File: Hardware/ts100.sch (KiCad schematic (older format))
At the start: 46 parts, among them J1 Jack-DC, J2 Iron+, J3 Iron-, J4 GND, J5 SWD, Q1 2SC3356, Q2 IRF4905STRLPBF, SW1 SW_Push, SW2 SW_Push, U1 AD823, U2 EUP3476, U3 1N4728A, U4 128x32 OLED, U5 STM32F103C8T6, Y1 8M

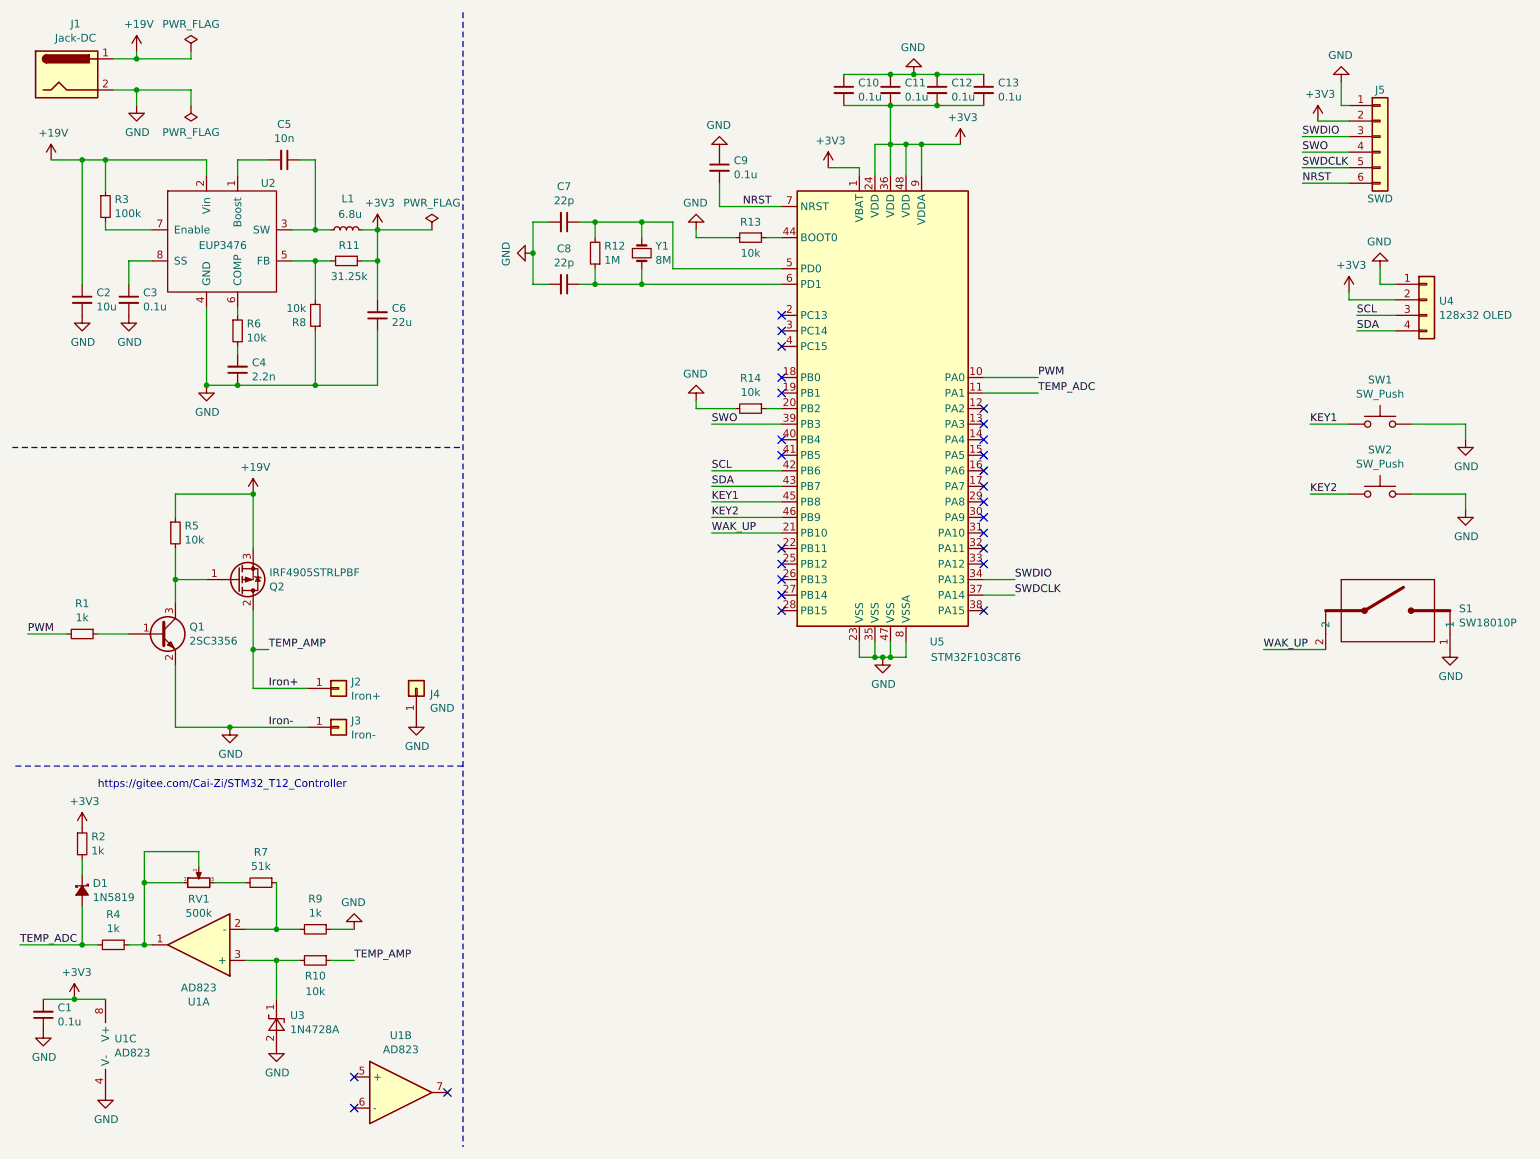
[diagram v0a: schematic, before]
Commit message: 修改原理图
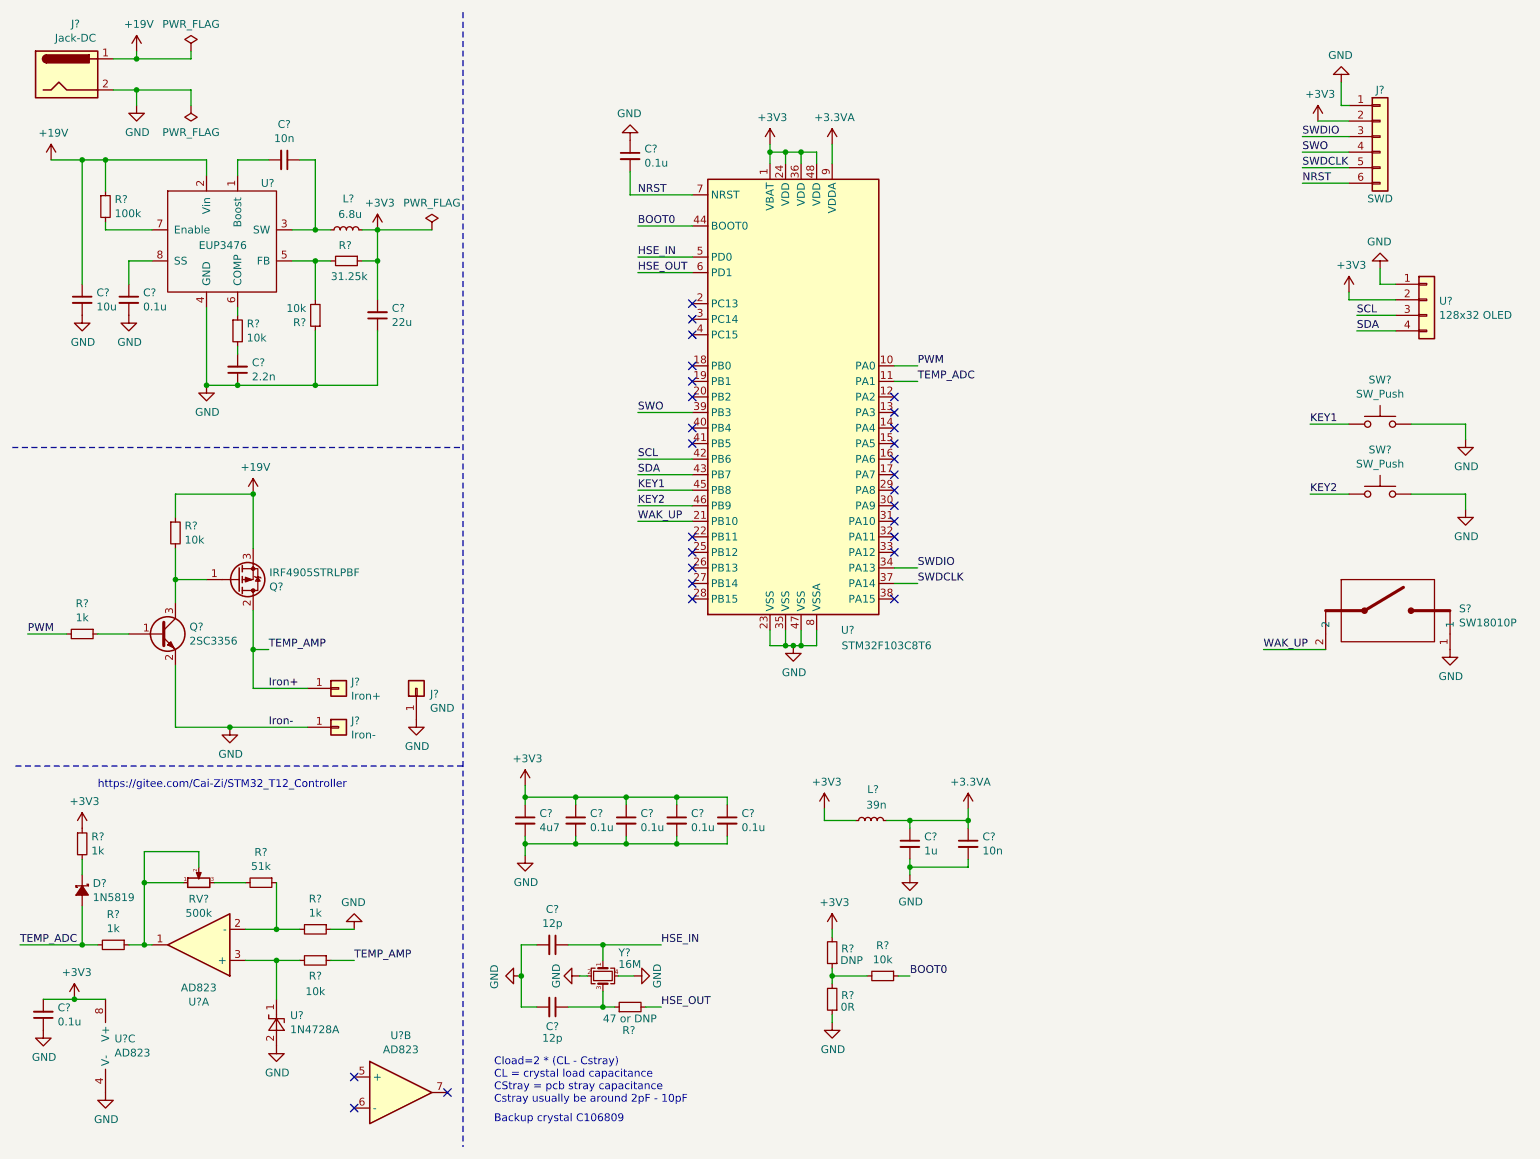
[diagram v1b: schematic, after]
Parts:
- removed R13: 10k, Resistor_SMD:R_0603_1608Metric, symbol Device:R_Small
- removed Y1: 8M, Crystal:Crystal_SMD_HC49-SD, symbol Device:Crystal_Small
- added C?: 4u7, Capacitor_SMD:C_0402_1005Metric, symbol Device:C_Small
- added C?: 1u, Capacitor_SMD:C_0402_1005Metric, symbol Device:C_Small
- added C?: 10n, Capacitor_SMD:C_0402_1005Metric, symbol Device:C_Small
- added L?: 39n, symbol Device:L_Small
- added R?: DNP, Resistor_SMD:R_0402_1005Metric, symbol Device:R_Small
- added R?: 0R, Resistor_SMD:R_0402_1005Metric, symbol Device:R_Small
- added Y?: 16M, Crystal:Crystal_SMD_3225-4Pin_3.2x2.5mm, symbol Device:Crystal_GND24_Small
- C?: renamed from C1; footprint Capacitor_SMD:C_0603_1608Metric -> Capacitor_SMD:C_0402_1005Metric
- C?: renamed from C7; value 22p -> 12p; footprint Capacitor_SMD:C_0603_1608Metric -> Capacitor_SMD:C_0402_1005Metric
- C?: renamed from C8; value 22p -> 12p; footprint Capacitor_SMD:C_0603_1608Metric -> Capacitor_SMD:C_0402_1005Metric
- C?: renamed from C10; footprint Capacitor_SMD:C_0603_1608Metric -> Capacitor_SMD:C_0402_1005Metric
- C?: renamed from C11; footprint Capacitor_SMD:C_0603_1608Metric -> Capacitor_SMD:C_0402_1005Metric
- C?: renamed from C12; footprint Capacitor_SMD:C_0603_1608Metric -> Capacitor_SMD:C_0402_1005Metric
- C?: renamed from C13; footprint Capacitor_SMD:C_0603_1608Metric -> Capacitor_SMD:C_0402_1005Metric
- R?: renamed from R2; footprint Resistor_SMD:R_0603_1608Metric -> Resistor_SMD:R_0402_1005Metric
- R?: renamed from R4; footprint Resistor_SMD:R_0603_1608Metric -> Resistor_SMD:R_0402_1005Metric
- R?: renamed from R7; footprint Resistor_SMD:R_0603_1608Metric -> Resistor_SMD:R_0402_1005Metric
- R?: renamed from R9; footprint Resistor_SMD:R_0603_1608Metric -> Resistor_SMD:R_0402_1005Metric
- R?: renamed from R10; footprint Resistor_SMD:R_0603_1608Metric -> Resistor_SMD:R_0402_1005Metric
- R?: renamed from R5; footprint Resistor_SMD:R_0603_1608Metric -> Resistor_SMD:R_0402_1005Metric
- R?: renamed from R1; footprint Resistor_SMD:R_0603_1608Metric -> Resistor_SMD:R_0402_1005Metric
- R?: renamed from R12; value 1M -> 47 or DNP; footprint Resistor_SMD:R_0603_1608Metric -> Resistor_SMD:R_0402_1005Metric
- R?: renamed from R14; footprint Resistor_SMD:R_0603_1608Metric -> Resistor_SMD:R_0402_1005Metric
- renumbered C2 to C?, C3 to C?, C5 to C?, C6 to C?, C4 to C?, C9 to C?, D1 to D?, J1 to J?, J2 to J?, J3 to J?, J4 to J?, J5 to J?, L1 to L?, Q2 to Q?, Q1 to Q?, R3 to R?, R11 to R?, R8 to R?, R6 to R?, RV1 to RV?, S1 to S?, SW1 to SW?, SW2 to SW?, U2 to U?, U3 to U?, U1 to U?, U5 to U?, U4 to U?
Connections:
- net +3V3: now also C?.1, C?.1, C?.1, C?.1, C?.1, L?.1, R?.2; no longer C?.2, C?.2, C?.2, C?.2, U?.9 (VDDA)
- net GND: now also C?.2, C?.2, C?.2, C?.2, C?.2, C?.2, C?.2, R?.1, Y?.2, Y?.4; no longer C?.1, C?.1, C?.1, C?.1, R?.2
- net BOOT0: now reaches U?.44 (BOOT0)
- net BOOT0: now also R?.1
- net at U?.20 (PB2): no longer R?.1
- net HSE_IN: now reaches C?.1, U?.5 (PD0)
- net HSE_IN: now also Y?.1; no longer R?.2
- net at C?.1, R?.1: now also Y?.3; no longer U?.6 (PD1)
- new net: R?.1, R?.2, R?.2
- new net +3.3VA: C?.1, C?.1, L?.2, U?.9 (VDDA)
- new net HSE_OUT: R?.2, U?.6 (PD1)
- no-connect marks 27 -> 28
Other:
- note added: "Backup crystal C106809"
- note added: "Cload=2 * (CL - Cstray)\nCL = crystal load capacitance\nCStray = pcb stray capacitance\nCstray usually be around 2pF - 10pF"
- moved on the sheet: C?, R?, U?
